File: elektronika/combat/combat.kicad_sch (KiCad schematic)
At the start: 35 parts, among them J1 odbiornik, J2 naped_prawy, J3 naped_lewy, J4 buzzer, J5 wyjscie do silnika +-, J6 Conn_02x04_Odd_Even, J7 zasilanie xt30, J8 Conn_01x01_Pin, J800 USB_C_Receptacle_USB2.0_16P, U1 ESP32-S3-WROOM-1, U2 kontroler_bldc, U3 AMS1117, U4 przetwornica

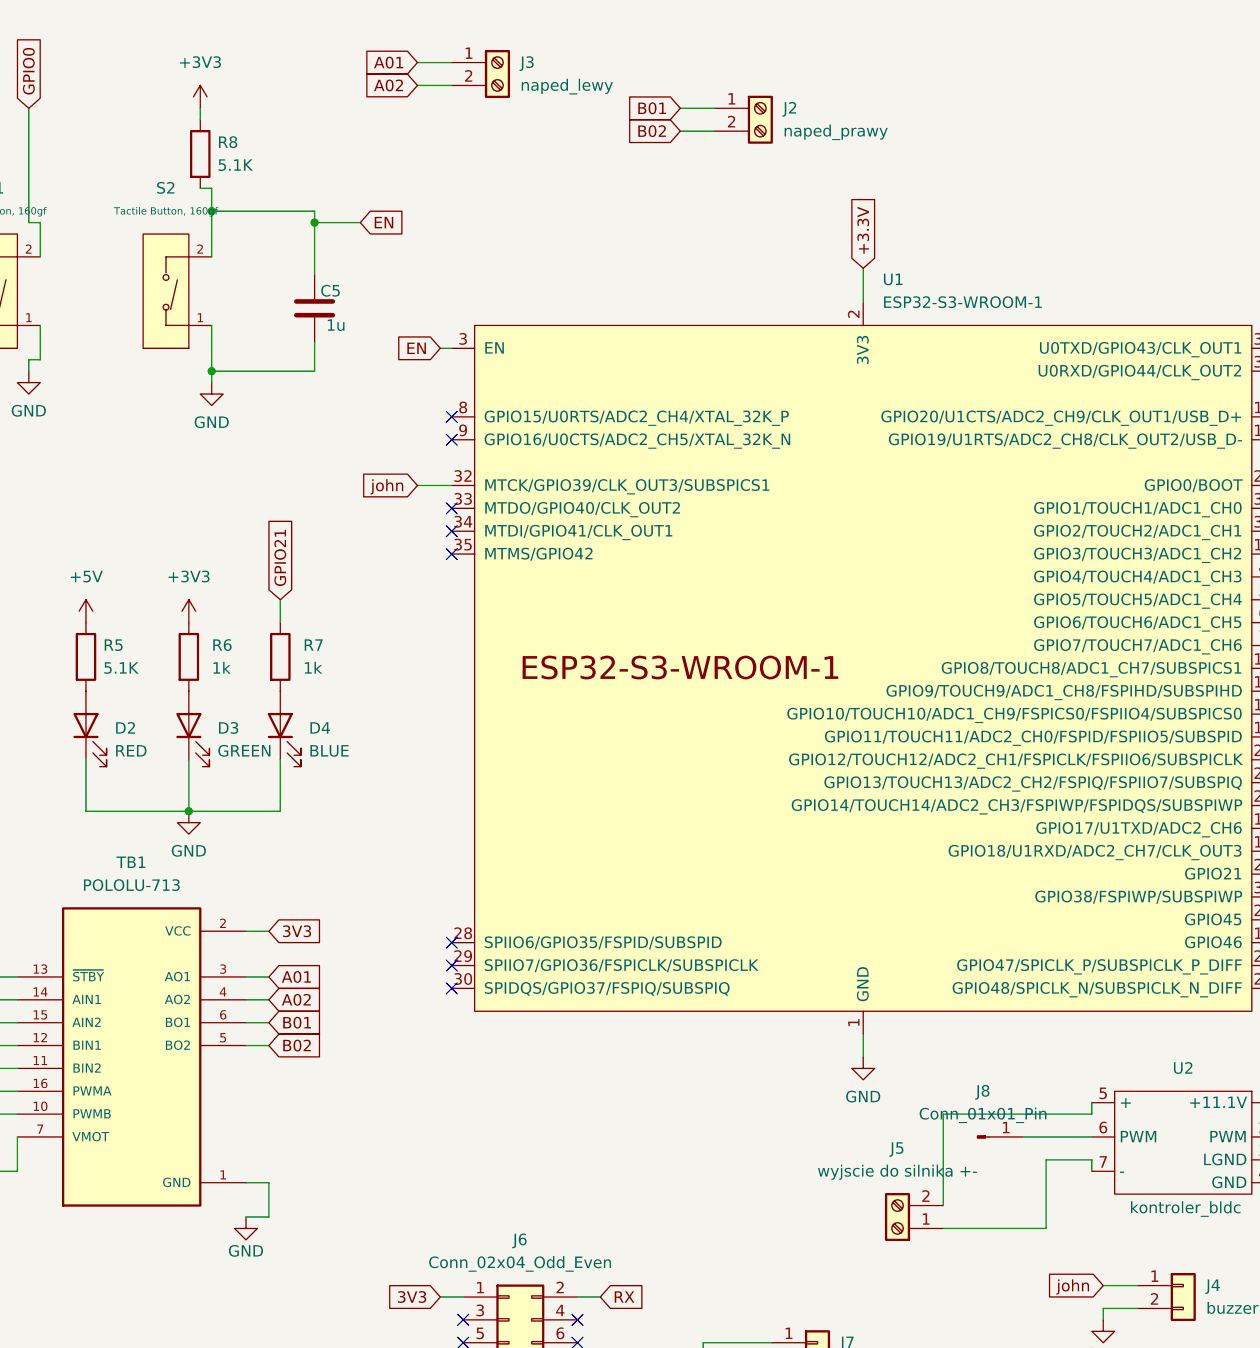
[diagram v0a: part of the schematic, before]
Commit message: pierwsze scieżki
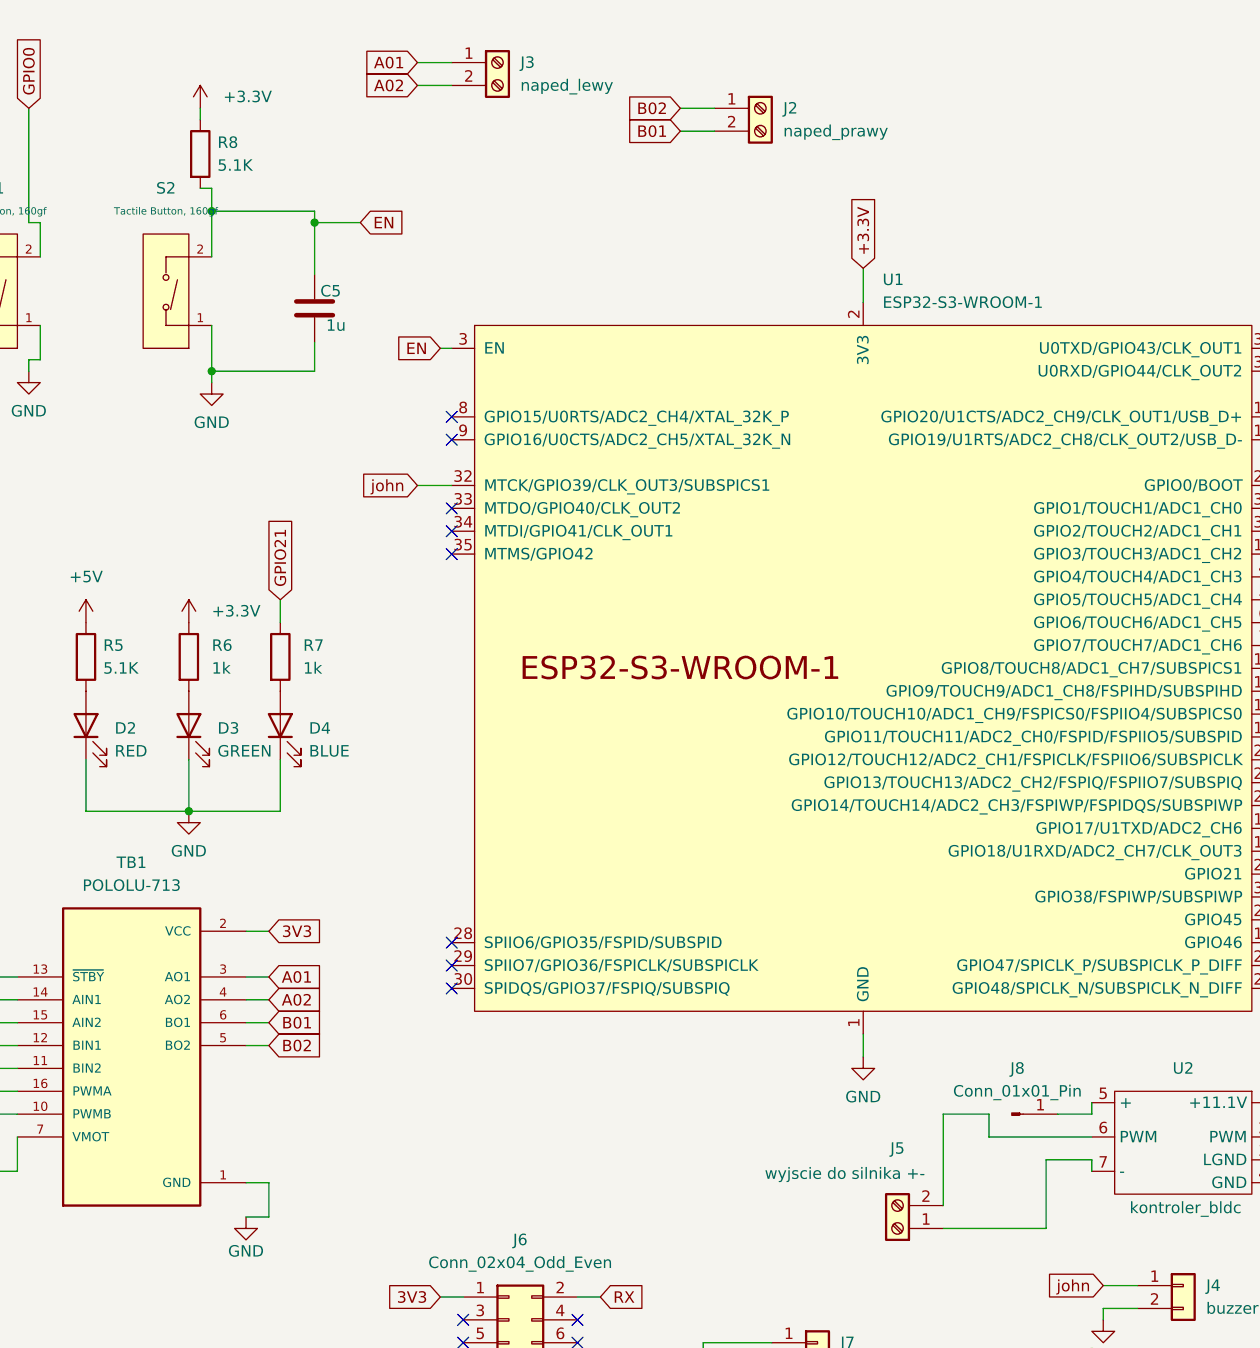
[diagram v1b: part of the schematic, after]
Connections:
- net +3V3 is gone; now on net +3.3V: R6.1, R8.1
- net B01: now also J2.2 (Pin_2); no longer J2.1 (Pin_1)
- net B02: now also J2.1 (Pin_1); no longer J2.2 (Pin_2)
- net at J5.2 (Pin_2): now also U2.6 (PWM); no longer U2.5 (+)
- net at J8.1 (Pin_1): now also U2.5 (+); no longer U2.6 (PWM)
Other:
- moved on the sheet: J8
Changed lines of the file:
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@@
 	(wire
 		(pts
+			(xy 99.06 36.83) (xy 102.87 36.83)
+		)
+		(stroke
+			(width 0)
+			(type default)
+		)
+	)
+	(wire
+		(pts
 			(xy 72.39 63.5) (xy 73.66 63.5)
 		)
@@
 	(wire
 		(pts
-			(xy 200.66 63.5) (xy 200.66 66.04)
+			(xy 128.27 148.59) (xy 133.35 148.59)
 		)
 		(stroke
@@
 	(wire
 		(pts
-			(xy 165.1 93.98) (xy 168.91 93.98)
+			(xy 200.66 63.5) (xy 200.66 66.04)
 		)
 		(stroke
@@
 	(wire
 		(pts
-			(xy 224.79 139.7) (xy 228.6 139.7)
+			(xy 165.1 93.98) (xy 168.91 93.98)
 		)
 		(stroke
@@
 	(wire
 		(pts
-			(xy 224.79 143.51) (xy 224.79 144.78)
+			(xy 224.79 139.7) (xy 228.6 139.7)
 		)
 		(stroke
@@
 	(wire
 		(pts
-			(xy 27.94 60.96) (xy 27.94 64.77)
+			(xy 224.79 143.51) (xy 224.79 144.78)
 		)
 		(stroke
@@
 	(wire
 		(pts
-			(xy 246.38 162.56) (xy 223.52 162.56)
+			(xy 133.35 151.13) (xy 144.78 151.13)
 		)
 		(stroke
@@
 	(wire
 		(pts
-			(xy 69.85 78.74) (xy 73.66 78.74)
+			(xy 27.94 60.96) (xy 27.94 64.77)
 		)
 		(stroke
@@
 	(wire
 		(pts
-			(xy 255.27 162.56) (xy 246.38 162.56)
+			(xy 246.38 162.56) (xy 223.52 162.56)
 		)
 		(stroke
@@
 	(wire
 		(pts
-			(xy 146.05 171.45) (xy 146.05 170.18)
+			(xy 69.85 78.74) (xy 73.66 78.74)
 		)
 		(stroke
@@
 	(wire
 		(pts
-			(xy 250.19 78.74) (xy 250.19 76.2)
+			(xy 255.27 162.56) (xy 246.38 162.56)
 		)
 		(stroke
@@
 	(wire
 		(pts
-			(xy 44.45 109.22) (xy 44.45 114.935)
+			(xy 146.05 171.45) (xy 146.05 170.18)
 		)
 		(stroke
@@
 	(wire
 		(pts
-			(xy 21.59 138.43) (xy 25.4 138.43)
+			(xy 250.19 78.74) (xy 250.19 76.2)
 		)
 		(stroke
@@
 	(wire
 		(pts
-			(xy 224.79 144.78) (xy 224.79 146.05)
+			(xy 44.45 109.22) (xy 44.45 114.935)
 		)
 		(stroke
@@
 	(wire
 		(pts
-			(xy 87.63 176.53) (xy 92.71 176.53)
+			(xy 21.59 138.43) (xy 25.4 138.43)
 		)
 		(stroke
@@
 	(wire
 		(pts
-			(xy 33.02 114.935) (xy 44.45 114.935)
+			(xy 224.79 144.78) (xy 224.79 146.05)
 		)
 		(stroke
@@
 	(wire
 		(pts
-			(xy 99.06 39.37) (xy 102.87 39.37)
+			(xy 133.35 148.59) (xy 133.35 151.13)
 		)
 		(stroke
@@
 	(wire
 		(pts
-			(xy 99.06 36.83) (xy 102.87 36.83)
+			(xy 87.63 176.53) (xy 92.71 176.53)
 		)
 		(stroke
@@
 	(wire
 		(pts
-			(xy 201.93 66.04) (xy 201.93 52.07)
+			(xy 33.02 114.935) (xy 44.45 114.935)
 		)
 		(stroke
@@
 	(wire
 		(pts
-			(xy 128.27 148.59) (xy 144.78 148.59)
+			(xy 201.93 66.04) (xy 201.93 52.07)
 		)
 		(stroke
@@
 	(wire
 		(pts
-			(xy 137.16 151.13) (xy 144.78 151.13)
-		)
-		(stroke
-			(width 0)
-			(type default)
-		)
-	)
-	(wire
-		(pts
 			(xy 255.27 130.81) (xy 255.27 134.62)
 		)
@@
 	(wire
 		(pts
+			(xy 99.06 39.37) (xy 102.87 39.37)
+		)
+		(stroke
+			(width 0)
+			(type default)
+		)
+	)
+	(wire
+		(pts
 			(xy 165.1 151.13) (xy 166.37 151.13)
 		)
@@
 	(wire
 		(pts
+			(xy 140.97 148.59) (xy 144.78 148.59)
+		)
+		(stroke
+			(width 0)
+			(type default)
+		)
+	)
+	(wire
+		(pts
 			(xy 261.62 107.95) (xy 262.89 107.95)
 		)
@@
 	(global_label "B02"
 		(shape input)
-		(at 99.06 39.37 180)
+		(at 99.06 36.83 180)
 		(fields_autoplaced yes)
 		(effects
@@
 		)
 		(property "Intersheetrefs" "${INTERSHEET_REFS}"
-			(at 92.3858 39.37 0)
+			(at 92.3858 36.83 0)
 			(hide yes)
 			(show_name no)
@@
 	(global_label "B01"
 		(shape input)
-		(at 99.06 36.83 180)
+		(at 99.06 39.37 180)
 		(fields_autoplaced yes)
 		(effects
@@
 		)
 		(property "Intersheetrefs" "${INTERSHEET_REFS}"
-			(at 92.3858 36.83 0)
+			(at 92.3858 39.37 0)
 			(hide yes)
 			(show_name no)
@@
 		(in_pos_files yes)
 		(dnp no)
-		(fields_autoplaced yes)
 		(property "Reference" "J5"
 			(at 123.19 152.4 0)
@@
 		)
 		(property "Value" "wyjscie do silnika +-"
-			(at 123.19 154.94 0)
+			(at 117.348 155.194 0)
 			(show_name no)
 			(do_not_autoplace no)
@@
 			)
 		)
-		(property "Value" "+3V3"
-			(at 44.45 88.9 0)
+		(property "Value" "+3.3V"
+			(at 46.99 92.7099 0)
 			(show_name no)
 			(do_not_autoplace no)
@@
 					(size 1.27 1.27)
 				)
+				(justify left)
 			)
 		)
@@
 			)
 		)
-		(property "Value" "+3V3"
-			(at 45.72 31.75 0)
+		(property "Value" "+3.3V"
+			(at 48.26 35.5599 0)
 			(show_name no)
 			(do_not_autoplace no)
@@
 					(size 1.27 1.27)
 				)
+				(justify left)
 			)
 		)
@@
 	(symbol
 		(lib_id "Connector:Conn_01x01_Pin")
-		(at 132.08 151.13 0)
+		(at 135.89 148.59 0)
 		(unit 1)
 		(body_style 1)
@@
 		(dnp no)
 		(property "Reference" "J8"
-			(at 132.715 146.05 0)
+			(at 136.525 143.51 0)
 			(show_name no)
 			(do_not_autoplace no)
@@
 		)
 		(property "Value" "Conn_01x01_Pin"
-			(at 132.715 148.59 0)
+			(at 136.525 146.05 0)
 			(show_name no)
 			(do_not_autoplace no)
@@
 		)
 		(property "Footprint" "Connector_PinHeader_2.54mm:PinHeader_1x01_P2.54mm_Vertical"
-			(at 138.176 165.862 0)
+			(at 141.986 163.322 0)
 			(hide yes)
 			(show_name no)
@@
 		)
 		(property "Datasheet" ""
-			(at 132.08 151.13 0)
+			(at 135.89 148.59 0)
 			(hide yes)
 			(show_name no)
@@
 		)
 		(property "Description" "Generic connector, single row, 01x01, script generated"
-			(at 132.08 151.13 0)
+			(at 135.89 148.59 0)
 			(hide yes)
 			(show_name no)

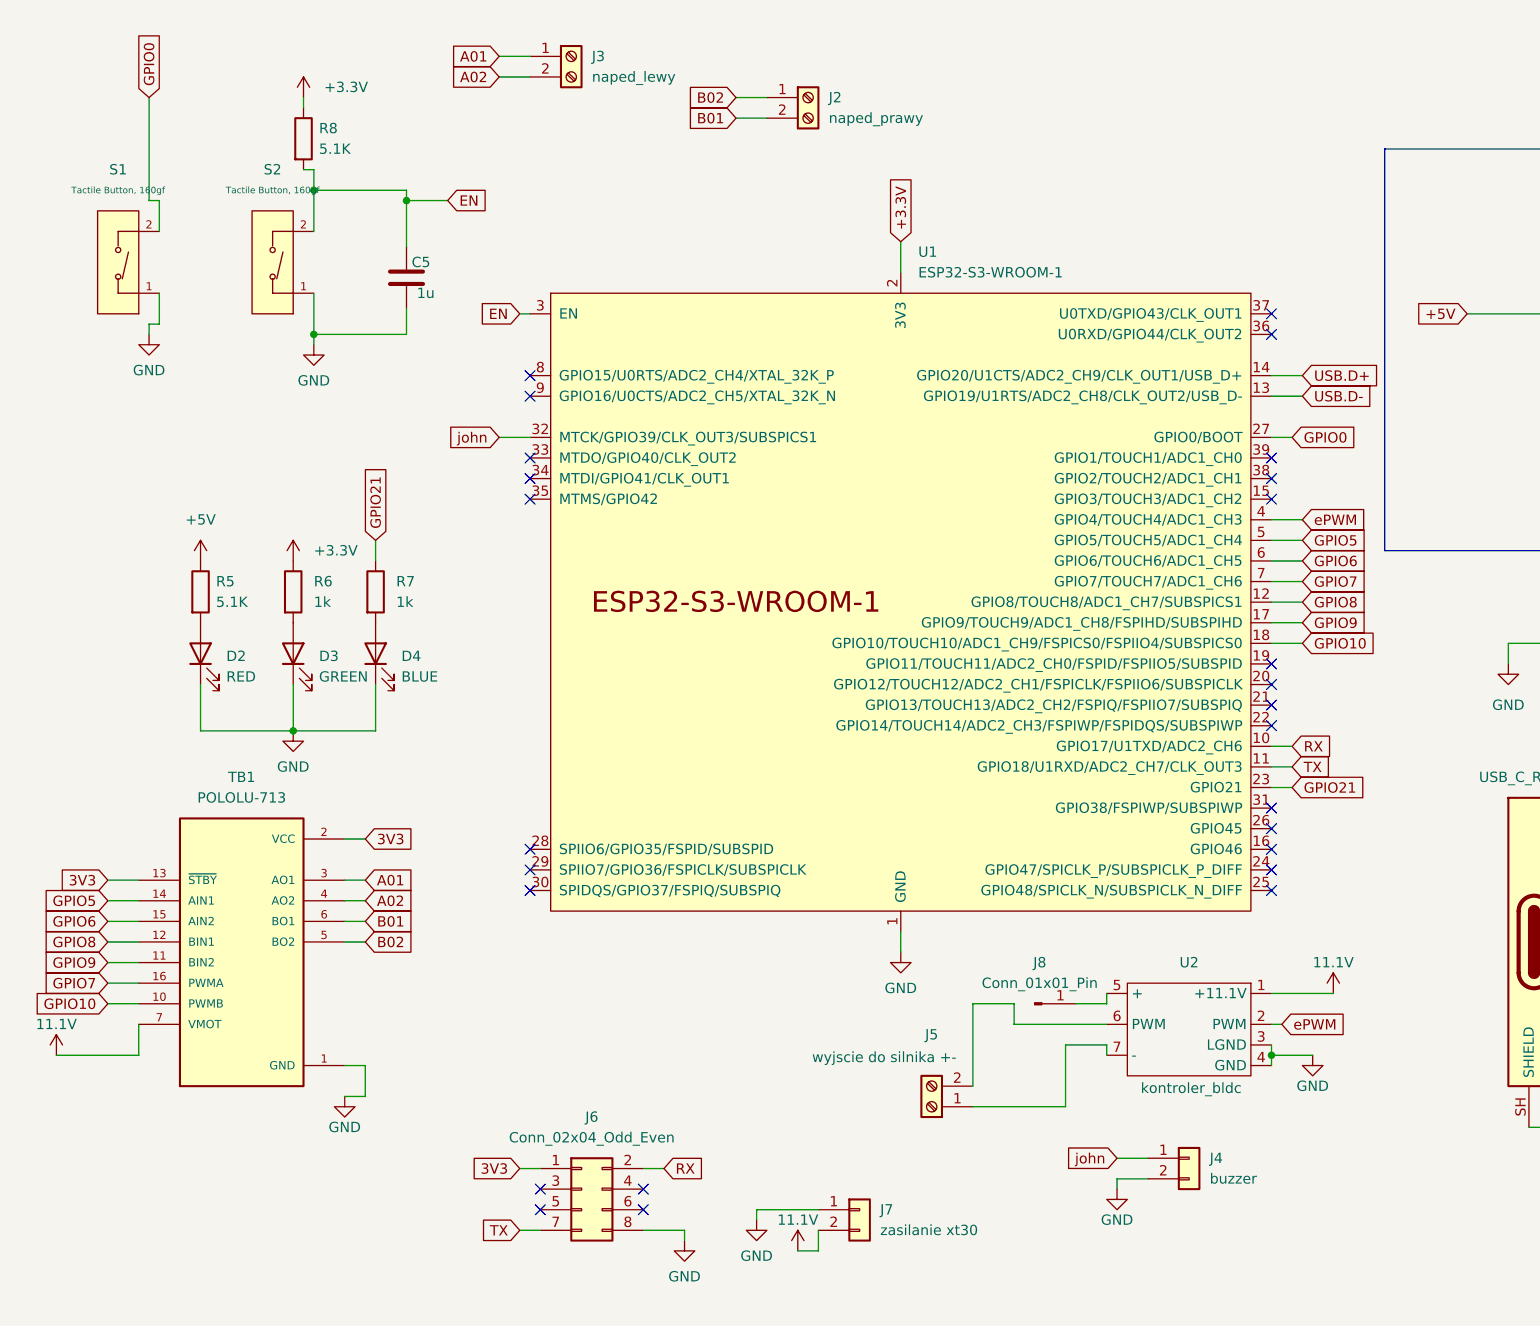
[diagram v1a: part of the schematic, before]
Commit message: PCB 1.0 complete
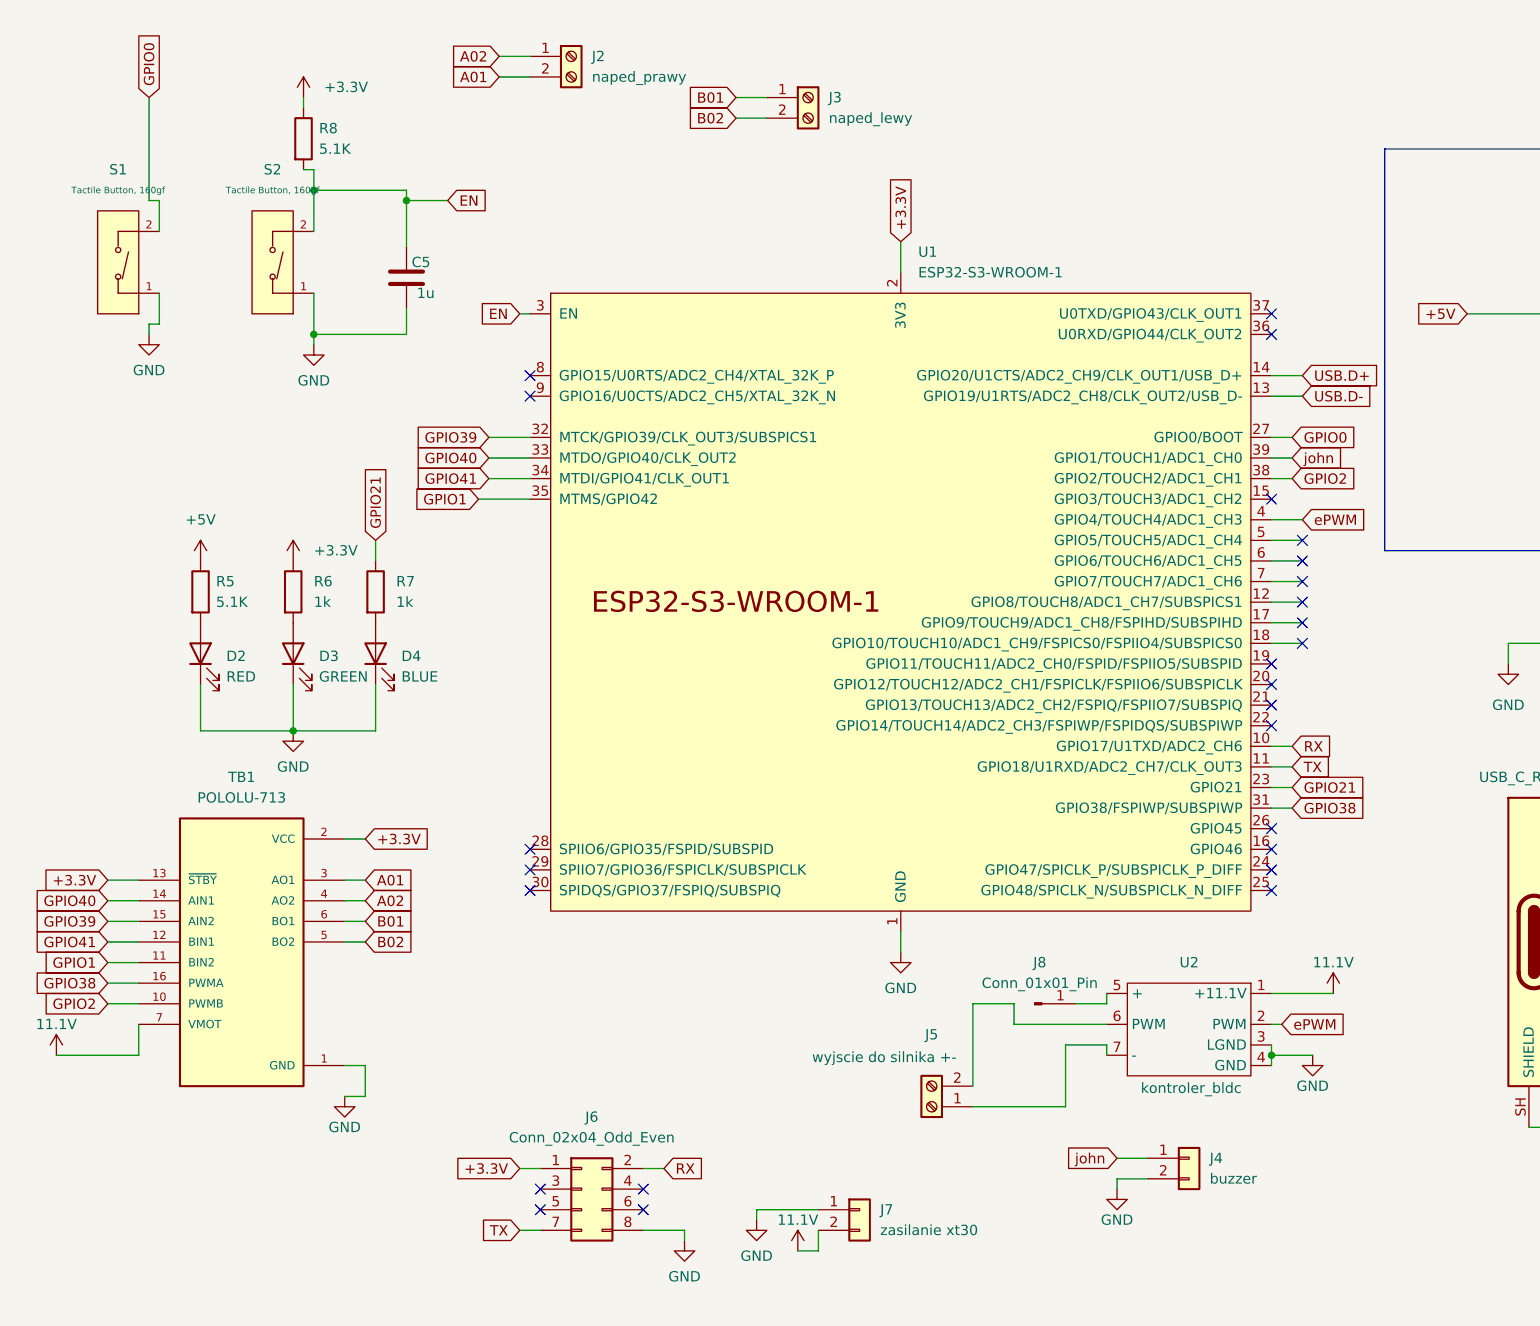
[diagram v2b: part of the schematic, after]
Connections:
- net 3V3 is gone; now on net +3.3V: J6.1 (Pin_1), TB1.13 (~{STBY}), TB1.2 (VCC)
- net A01: now also J2.2 (Pin_2); no longer J3.1 (Pin_1)
- net A02: now also J2.1 (Pin_1); no longer J3.2 (Pin_2)
- net B01: now also J3.1 (Pin_1); no longer J2.2 (Pin_2)
- net B02: now also J3.2 (Pin_2); no longer J2.1 (Pin_1)
- net john: now also U1.39 (GPIO1/TOUCH1/ADC1_CH0); no longer U1.32 (MTCK/GPIO39/CLK_OUT3/SUBSPICS1)
- net GPIO38: now reaches U1.31 (GPIO38/FSPIWP/SUBSPIWP)
- net GPIO38: now also TB1.16 (PWMA)
- net GPIO40: now reaches U1.33 (MTDO/GPIO40/CLK_OUT2)
- net GPIO40: now also TB1.14 (AIN1)
- net GPIO41: now reaches U1.34 (MTDI/GPIO41/CLK_OUT1)
- net GPIO41: now also TB1.12 (BIN1)
- net GPIO1: now reaches U1.35 (MTMS/GPIO42)
- net GPIO1: now also TB1.11 (BIN2)
- net GPIO2: now reaches U1.38 (GPIO2/TOUCH2/ADC1_CH1)
- net GPIO2: now also TB1.10 (PWMB)
- net GPIO10: no longer names the net of U1.18 (GPIO10/TOUCH10/ADC1_CH9/FSPICS0/FSPIIO4/SUBSPICS0)
- net GPIO10: no longer TB1.10 (PWMB)
- net GPIO5: no longer names the net of U1.5 (GPIO5/TOUCH5/ADC1_CH4)
- net GPIO5: no longer TB1.14 (AIN1)
- net GPIO6: no longer names the net of U1.6 (GPIO6/TOUCH6/ADC1_CH5)
- net GPIO6: no longer TB1.15 (AIN2)
- net GPIO7: no longer names the net of U1.7 (GPIO7/TOUCH7/ADC1_CH6)
- net GPIO7: no longer TB1.16 (PWMA)
- net GPIO8: no longer names the net of U1.12 (GPIO8/TOUCH8/ADC1_CH7/SUBSPICS1)
- net GPIO8: no longer TB1.12 (BIN1)
- net GPIO9: no longer names the net of U1.17 (GPIO9/TOUCH9/ADC1_CH8/FSPIHD/SUBSPIHD)
- net GPIO9: no longer TB1.11 (BIN2)
- new net GPIO39: TB1.15 (AIN2), U1.32 (MTCK/GPIO39/CLK_OUT3/SUBSPICS1)
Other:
- moved on the sheet: J2, J3
